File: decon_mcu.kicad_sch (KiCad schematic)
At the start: 56 parts, among them J1 Conn_01x02, J10 Conn_01x04, J11 Conn_01x06, J12 Conn_01x06, J13 Conn_01x04, J14 Conn_01x16, J15 Conn_01x16, J16 Conn_01x16, J17 Conn_01x16, J18 Conn_01x04, J2 GPIO, J3 Conn_01x06, J4 Conn_01x06, J5 FLASH, J6 Conn_01x06, J7 Conn_01x05, J8 Conn_01x06, J9 Conn_01x06, SW1 SW_Push, SW2 SW_Push, U1 URB2405YMD-10WR3, U2 AZ1117-3.3, U3 STM32F401R_B-C_Tx, Y1 Crystal, Y2 Crystal_GND24

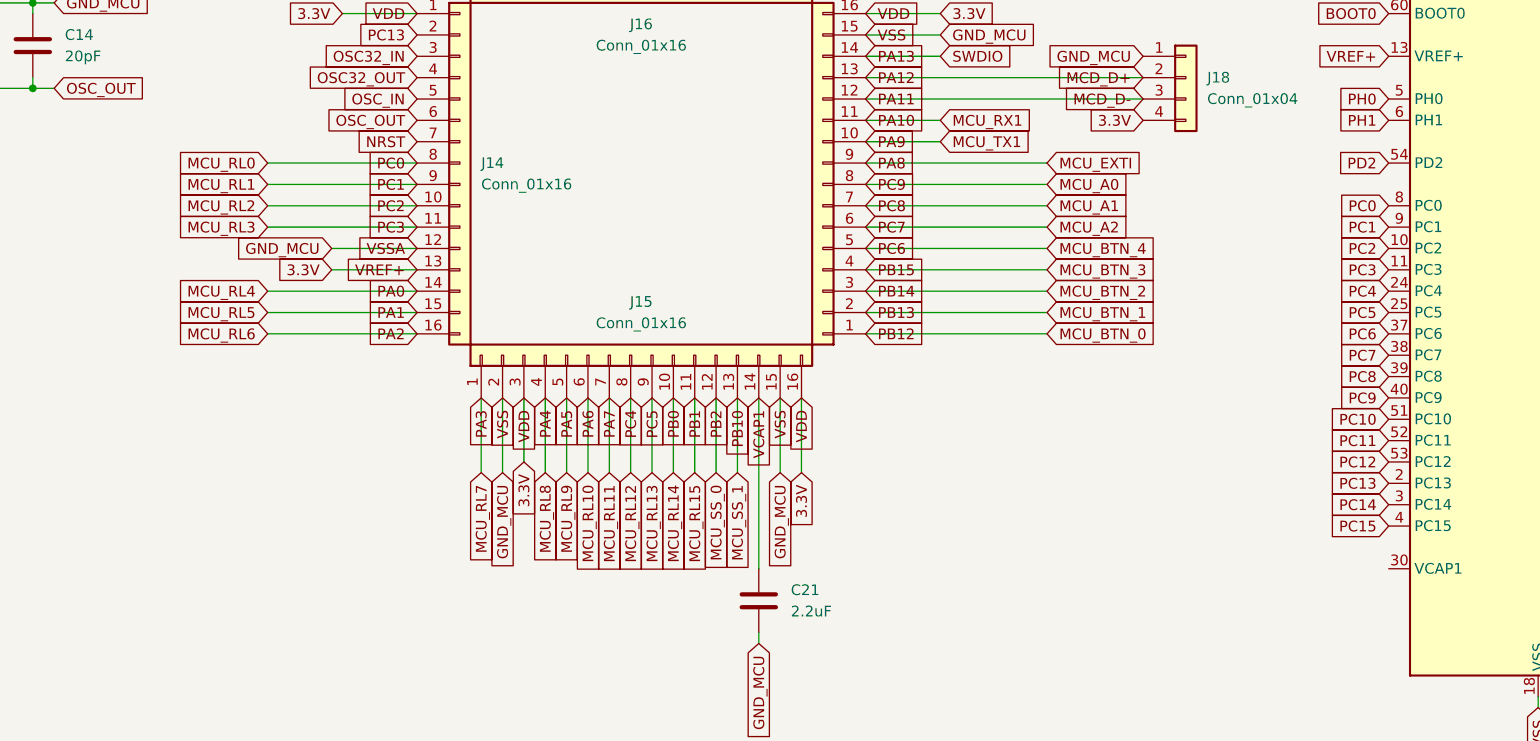
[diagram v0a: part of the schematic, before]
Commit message: modified:   DECON_Ctrl_Panel.kicad_pcb
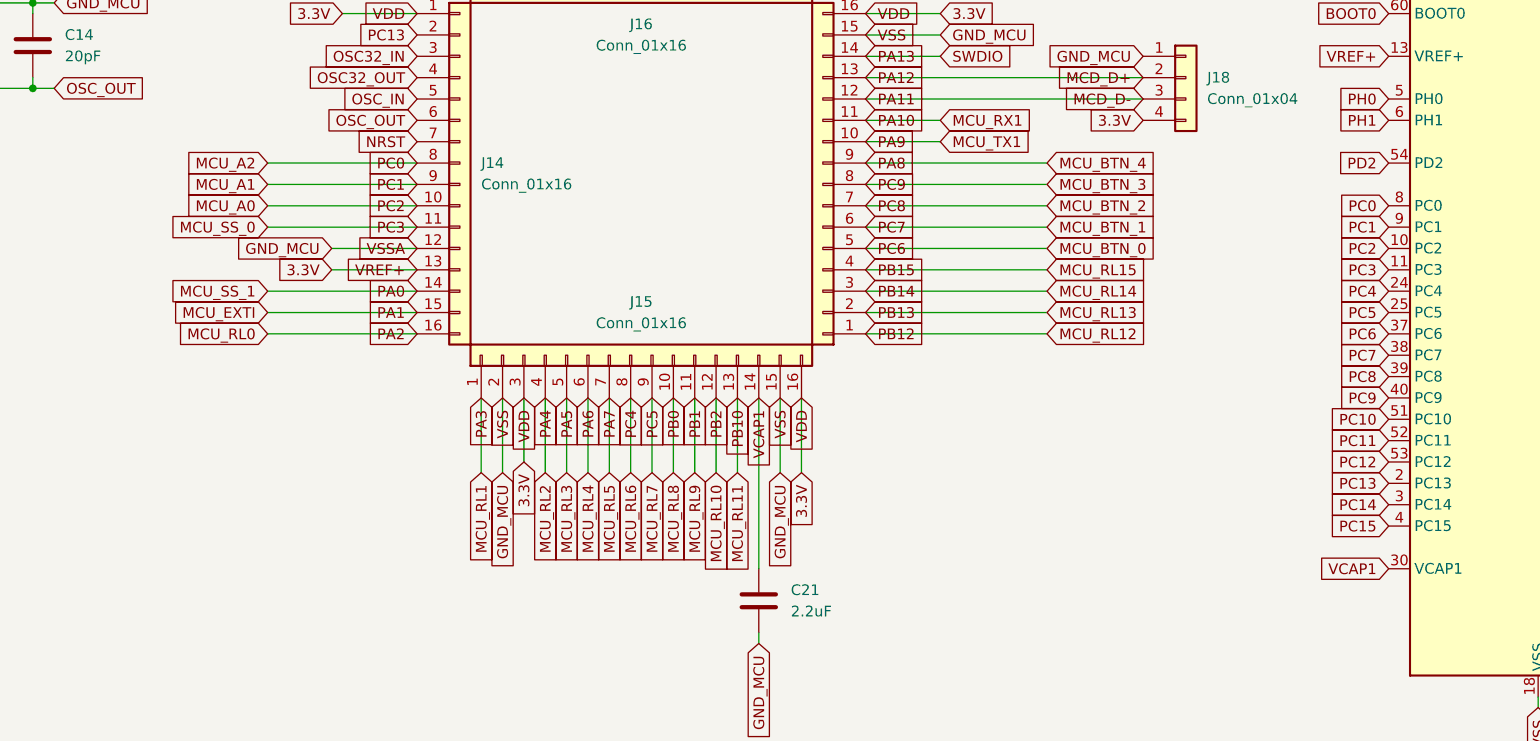
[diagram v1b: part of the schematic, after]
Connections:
- net MCU_A0: now also J14.10 (Pin_10), U3.10 (PC2); no longer J17.8 (Pin_8), U3.40 (PC9)
- net MCU_A1: now also J14.9 (Pin_9), U3.9 (PC1); no longer J17.7 (Pin_7), U3.39 (PC8)
- net MCU_A2: now also J14.8 (Pin_8), U3.8 (PC0); no longer J17.6 (Pin_6), U3.38 (PC7)
- net MCU_BTN_0: now also J17.5 (Pin_5), U3.37 (PC6); no longer J17.1 (Pin_1), U3.33 (PB12)
- net MCU_BTN_1: now also J17.6 (Pin_6), U3.38 (PC7); no longer J17.2 (Pin_2), U3.34 (PB13)
- net MCU_BTN_2: now also J17.7 (Pin_7), U3.39 (PC8); no longer J17.3 (Pin_3), U3.35 (PB14)
- net MCU_BTN_3: now also J17.8 (Pin_8), U3.40 (PC9); no longer J17.4 (Pin_4), U3.36 (PB15)
- net MCU_BTN_4: now also C2.1, J17.9 (Pin_9), R2.2, SW1.1, U3.41 (PA8); no longer J17.5 (Pin_5), U3.37 (PC6)
- net MCU_EXTI: now also J14.15 (Pin_15), U3.15 (PA1); no longer C2.1, J17.9 (Pin_9), R2.2, SW1.1, U3.41 (PA8)
- net MCU_RL0: now also J14.16 (Pin_16), U3.16 (PA2); no longer J14.8 (Pin_8), U3.8 (PC0)
- net MCU_RL1: now also J15.1 (Pin_1), U3.17 (PA3); no longer J14.9 (Pin_9), U3.9 (PC1)
- net MCU_RL10: now also J15.12 (Pin_12), U3.28 (PB2); no longer J15.6 (Pin_6), U3.22 (PA6)
- net MCU_RL11: now also J15.13 (Pin_13), U3.29 (PB10); no longer J15.7 (Pin_7), U3.23 (PA7)
- net MCU_RL12: now also J17.1 (Pin_1), U3.33 (PB12); no longer J15.8 (Pin_8), U3.24 (PC4)
- net MCU_RL13: now also J17.2 (Pin_2), U3.34 (PB13); no longer J15.9 (Pin_9), U3.25 (PC5)
- net MCU_RL14: now also J17.3 (Pin_3), U3.35 (PB14); no longer J15.10 (Pin_10), U3.26 (PB0)
- net MCU_RL15: now also J17.4 (Pin_4), U3.36 (PB15); no longer J15.11 (Pin_11), U3.27 (PB1)
- net MCU_RL2: now also J15.4 (Pin_4), U3.20 (PA4); no longer J14.10 (Pin_10), U3.10 (PC2)
- net MCU_RL3: now also J15.5 (Pin_5), U3.21 (PA5); no longer J14.11 (Pin_11), U3.11 (PC3)
- net MCU_RL4: now also J15.6 (Pin_6), U3.22 (PA6); no longer J14.14 (Pin_14), U3.14 (PA0)
- net MCU_RL5: now also J15.7 (Pin_7), U3.23 (PA7); no longer J14.15 (Pin_15), U3.15 (PA1)
- net MCU_RL6: now also J15.8 (Pin_8), U3.24 (PC4); no longer J14.16 (Pin_16), U3.16 (PA2)
- net MCU_RL7: now also J15.9 (Pin_9), U3.25 (PC5); no longer J15.1 (Pin_1), U3.17 (PA3)
- net MCU_RL8: now also J15.10 (Pin_10), U3.26 (PB0); no longer J15.4 (Pin_4), U3.20 (PA4)
- net MCU_RL9: now also J15.11 (Pin_11), U3.27 (PB1); no longer J15.5 (Pin_5), U3.21 (PA5)
- net MCU_SS_0: now also J14.11 (Pin_11), U3.11 (PC3); no longer J15.12 (Pin_12), U3.28 (PB2)
- net MCU_SS_1: now also J14.14 (Pin_14), U3.14 (PA0); no longer J15.13 (Pin_13), U3.29 (PB10)
- net VCAP1: now also U3.30 (VCAP1)
